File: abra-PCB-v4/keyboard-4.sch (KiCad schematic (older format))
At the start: 294 parts, among them J2 Conn_01x04, Q1 Q_NPN_BCE, SW1 Rotary_Encoder_Switch, SW2 SW_Push, U1 ATmega32U4-AU, U2 PRTR5V0U2X, Y1 16MHz

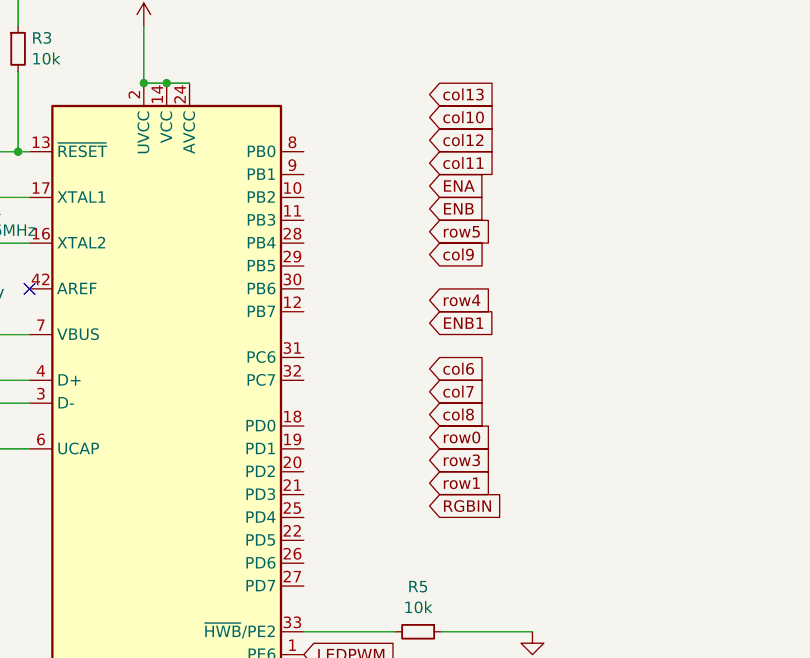
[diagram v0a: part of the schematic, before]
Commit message: version 4
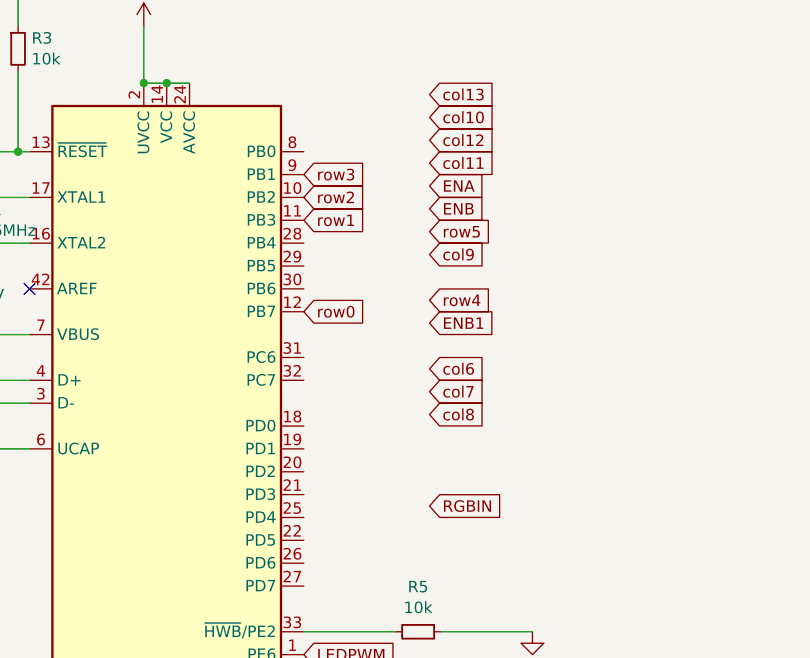
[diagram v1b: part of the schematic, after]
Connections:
- net row0: now also U1.12 (PB7)
- net row1: now also U1.11 (PB3)
- net row2: now also U1.10 (PB2)
- net row3: now also U1.9 (PB1)
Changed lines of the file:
@@
 EESchema Schematic File Version 4
+LIBS:keyboard-4-cache
 EELAYER 30 0
 EELAYER END
@@
 col8
 NoConn ~ 1750 5800
-Text GLabel 3500 6450 2    50   Input ~ 0
+Text GLabel 2950 5900 2    50   Input ~ 0
 row0
 Wire Wire Line
 	1600 4900 1600 5200
-Text GLabel 3500 6650 2    50   Input ~ 0
+Text GLabel 2950 5500 2    50   Input ~ 0
 row1
-Text GLabel 3500 6550 2    50   Input ~ 0
+Text GLabel 2950 5300 2    50   Input ~ 0
 row3
 Text GLabel 3500 5850 2    50   Input ~ 0
@@
 Text GLabel 3500 6750 2    50   Input ~ 0
 RGBIN
+Text GLabel 2950 5400 2    50   Input ~ 0
+row2
 $EndSCHEMATC

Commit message: v4 routing complete
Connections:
- net ENB1 is gone; now on net col14: K_28.1 (COL), K_43.1 (COL), K_58.1 (COL), K_71.1 (COL), K_82.1 (COL), SW1.S1
- net ENA: now also U1.19 (PD1)
- net ENB: now also U1.20 (PD2)
- net RGBIN: now also U1.41 (PF0)
- net col0: now also U1.40 (PF1)
- net col1: now also U1.39 (PF4)
- net col10: now also U1.27 (PD7)
- net col11: now also U1.26 (PD6)
- net col12: now also U1.25 (PD4)
- net col13: now also U1.22 (PD5)
- net col2: now also U1.38 (PF5)
- net col3: now also U1.37 (PF6)
- net col4: now also U1.36 (PF7)
- net col5: now also U1.32 (PC7)
- net col6: now also U1.31 (PC6)
- net col7: now also U1.30 (PB6)
- net col8: now also U1.29 (PB5)
- net col9: now also U1.28 (PB4)
- net row0: now also U1.8 (PB0); no longer U1.12 (PB7)
- net row1: now also U1.9 (PB1); no longer U1.11 (PB3)
- net row3: now also U1.11 (PB3); no longer U1.9 (PB1)
- net row4: now also U1.12 (PB7)
- net row5: now also U1.18 (PD0)
- net col14: now reaches U1.21 (PD3)
- net ENB2: no longer names the net of D_13.2 (A), SW1.S2
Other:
- moved on the sheet: D_13, SW1
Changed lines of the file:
@@
 EESchema Schematic File Version 4
-LIBS:keyboard-4-cache
 EELAYER 30 0
 EELAYER END
@@
 Connection ~ 20550 1300
 Connection ~ 20100 1750
-Text GLabel 21550 1000 0    50   Input ~ 0
+Text GLabel 21550 850  0    50   Input ~ 0
 col14
-Wire Wire Line
-	21550 1000 21550 1300
-$Comp
-L Device:D_Small D_13
-U 1 1 00000130
-P 21100 1650
-F 0 "D_13" V 21170 1550 50  0000 R CNN
-F 1 "D" V 21080 1550 50  0000 R CNN
-F 2 "Diode_SMD:D_SOD-123" H 20800 1600 50  0001 C CNN
-F 3 "~" H 20800 1600 50  0001 C CNN
-	1    21100 1650
-	0    -1   -1   0
-$EndComp
-Wire Wire Line
-	21300 1300 21550 1300
-Wire Wire Line
-	21100 1500 21100 1550
-Connection ~ 21550 1300
 Text GLabel 6650 2750 0    50   Input ~ 0
 row1
@@
 Wire Wire Line
 	21100 2500 21100 2550
-Connection ~ 21550 2300
 Text GLabel 6650 3750 0    50   Input ~ 0
 row2
@@
 	19100 1750 20100 1750
 Wire Wire Line
-	20100 1750 21100 1750
-Wire Wire Line
 	8100 2750 9100 2750
 Wire Wire Line
@@
 	20550 1300 20550 2300
 Wire Wire Line
-	21550 1300 21550 2300
-Wire Wire Line
 	12100 1750 13100 1750
 Wire Wire Line
@@
 L Device:Rotary_Encoder_Switch SW1
 U 1 1 5F2411FE
-P 21700 8600
-F 0 "SW1" H 21700 8967 50  0000 C CNN
-F 1 "Rotary_Encoder_Switch" H 21700 8876 50  0000 C CNN
-F 2 "Rotary_Encoder:RotaryEncoder_Alps_EC11E-Switch_Vertical_H20mm" H 21550 8760 50  0001 C CNN
-F 3 "~" H 21700 8860 50  0001 C CNN
-	1    21700 8600
-	1    0    0    -1
-$EndComp
-Text GLabel 22000 8700 2    50   Input ~ 0
-ENB2
-Text GLabel 22000 8500 2    50   Input ~ 0
-ENB1
-Text GLabel 21300 1300 0    50   Input ~ 0
-ENB1
-Text GLabel 21100 1500 0    50   Input ~ 0
-ENB2
+P 21250 1250
+F 0 "SW1" H 21250 1617 50  0000 C CNN
+F 1 "Rotary_Encoder_Switch" H 21250 1526 50  0000 C CNN
+F 2 "Rotary_Encoder:RotaryEncoder_Alps_EC11E-Switch_Vertical_H20mm" H 21100 1410 50  0001 C CNN
+F 3 "~" H 21250 1510 50  0001 C CNN
+	1    21250 1250
+	1    0    0    -1
+$EndComp
 Wire Wire Line
 	6900 4000 7400 4000
@@
 Connection ~ 9050 10400
 Connection ~ 9450 10400
-Text GLabel 3450 8500 2    50   Input ~ 0
+Text GLabel 2950 7700 2    50   Input ~ 0
 col0
-Text GLabel 3450 8400 2    50   Input ~ 0
+Text GLabel 2950 7800 2    50   Input ~ 0
 col1
-Text GLabel 3450 8300 2    50   Input ~ 0
+Text GLabel 2950 7900 2    50   Input ~ 0
 col2
-Text GLabel 3450 8200 2    50   Input ~ 0
+Text GLabel 2950 8000 2    50   Input ~ 0
 col3
-Text GLabel 3450 8100 2    50   Input ~ 0
+Text GLabel 2950 8100 2    50   Input ~ 0
 col4
-Text GLabel 3450 8000 2    50   Input ~ 0
+Text GLabel 2950 6200 2    50   Input ~ 0
 col5
 Connection ~ 7100 4500
@@
 Connection ~ 7250 4350
 Connection ~ 8250 4350
-Text GLabel 3500 5950 2    50   Input ~ 0
-ENB1
-Text GLabel 3500 4950 2    50   Input ~ 0
+Text GLabel 2950 6900 2    50   Input ~ 0
 col13
-Text GLabel 3500 5150 2    50   Input ~ 0
+Text GLabel 2950 6800 2    50   Input ~ 0
 col12
-Text GLabel 3500 5050 2    50   Input ~ 0
+Text GLabel 2950 7100 2    50   Input ~ 0
 col10
 $Comp
@@
 	1    0    0    -1
 $EndComp
-Text GLabel 3500 6150 2    50   Input ~ 0
+Text GLabel 2950 6100 2    50   Input ~ 0
 col6
-Text GLabel 3500 6250 2    50   Input ~ 0
+Text GLabel 2950 5800 2    50   Input ~ 0
 col7
-Text GLabel 3500 6350 2    50   Input ~ 0
+Text GLabel 2950 5700 2    50   Input ~ 0
 col8
 NoConn ~ 1750 5800
-Text GLabel 2950 5900 2    50   Input ~ 0
+Text GLabel 2950 5200 2    50   Input ~ 0
 row0
 Wire Wire Line
 	1600 4900 1600 5200
-Text GLabel 2950 5500 2    50   Input ~ 0
-row1
 Text GLabel 2950 5300 2    50   Input ~ 0
+row1
+Text GLabel 2950 5500 2    50   Input ~ 0
 row3
-Text GLabel 3500 5850 2    50   Input ~ 0
+Text GLabel 2950 5900 2    50   Input ~ 0
 row4
-Text GLabel 3500 5550 2    50   Input ~ 0
+Text GLabel 2950 6400 2    50   Input ~ 0
 row5
-Text GLabel 21400 8500 0    50   Input ~ 0
+Text GLabel 20950 1150 0    50   Input ~ 0
 ENA
-Text GLabel 21400 8700 0    50   Input ~ 0
+Text GLabel 20950 1350 0    50   Input ~ 0
 ENB
 Wire Wire Line
-	21400 8600 21100 8600
+	20950 1250 20650 1250
 $Comp
 L power:GND #PWR0120
 U 1 1 5FBF5950
-P 21100 8600
-F 0 "#PWR0120" H 21100 8350 50  0001 C CNN
-F 1 "GND" H 21105 8427 50  0000 C CNN
-F 2 "" H 21100 8600 50  0001 C CNN
-F 3 "" H 21100 8600 50  0001 C CNN
-	1    21100 8600
+P 20650 1250
+F 0 "#PWR0120" H 20650 1000 50  0001 C CNN
+F 1 "GND" H 20655 1077 50  0000 C CNN
+F 2 "" H 20650 1250 50  0001 C CNN
+F 3 "" H 20650 1250 50  0001 C CNN
+	1    20650 1250
 	1    0    0    -1
 $EndComp
-Text GLabel 3500 5350 2    50   Input ~ 0
+Text GLabel 2950 6500 2    50   Input ~ 0
 ENA
-Text GLabel 3500 5450 2    50   Input ~ 0
+Text GLabel 2950 6600 2    50   Input ~ 0
 ENB
 Text GLabel 2950 7400 2    50   Input ~ 0
 LEDPWM
-Text GLabel 3500 5650 2    50   Input ~ 0
+Text GLabel 2950 5600 2    50   Input ~ 0
 col9
-Text GLabel 3500 5250 2    50   Input ~ 0
+Text GLabel 2950 7000 2    50   Input ~ 0
 col11
-Text GLabel 3500 6750 2    50   Input ~ 0
+Text GLabel 2950 7600 2    50   Input ~ 0
 RGBIN
 Text GLabel 2950 5400 2    50   Input ~ 0
 row2
+Text GLabel 2950 6700 2    50   Input ~ 0
+col14
+$Comp
+L Device:D_Small D_13
+U 1 1 00000130
+P 21550 1650
+F 0 "D_13" V 21620 1550 50  0000 R CNN
+F 1 "D" V 21530 1550 50  0000 R CNN
+F 2 "Diode_SMD:D_SOD-123" H 21250 1600 50  0001 C CNN
+F 3 "~" H 21250 1600 50  0001 C CNN
+	1    21550 1650
+	0    -1   -1   0
+$EndComp
+Wire Wire Line
+	20100 1750 21550 1750
+Wire Wire Line
+	21550 1350 21550 1550
+Wire Wire Line
+	21550 2300 21750 2300
+Wire Wire Line
+	21750 2300 21750 1200
+Wire Wire Line
+	21750 1200 21550 1200
+Wire Wire Line
+	21550 1200 21550 1150
+Connection ~ 21550 2300
+Connection ~ 21550 1150
+Wire Wire Line
+	21550 1150 21550 850
 $EndSCHEMATC
